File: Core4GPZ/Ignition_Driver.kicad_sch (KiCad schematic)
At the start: 8 parts, among them Q1 IRF740, Q2 IRF740

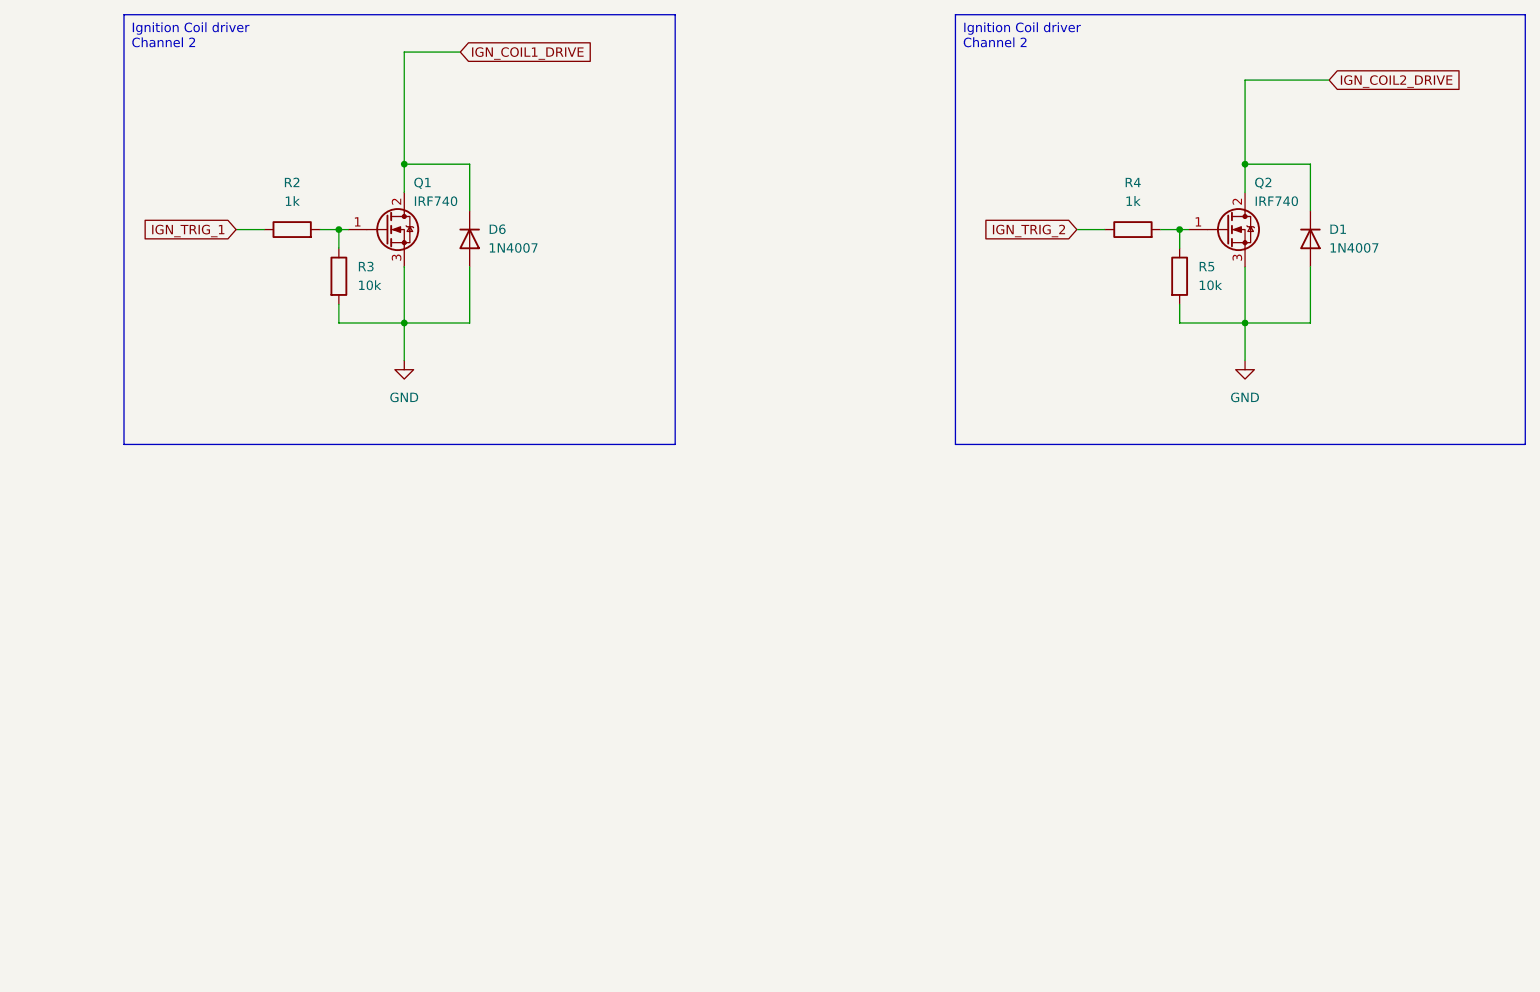
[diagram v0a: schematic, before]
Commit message: Test montage générateur de Haute tension
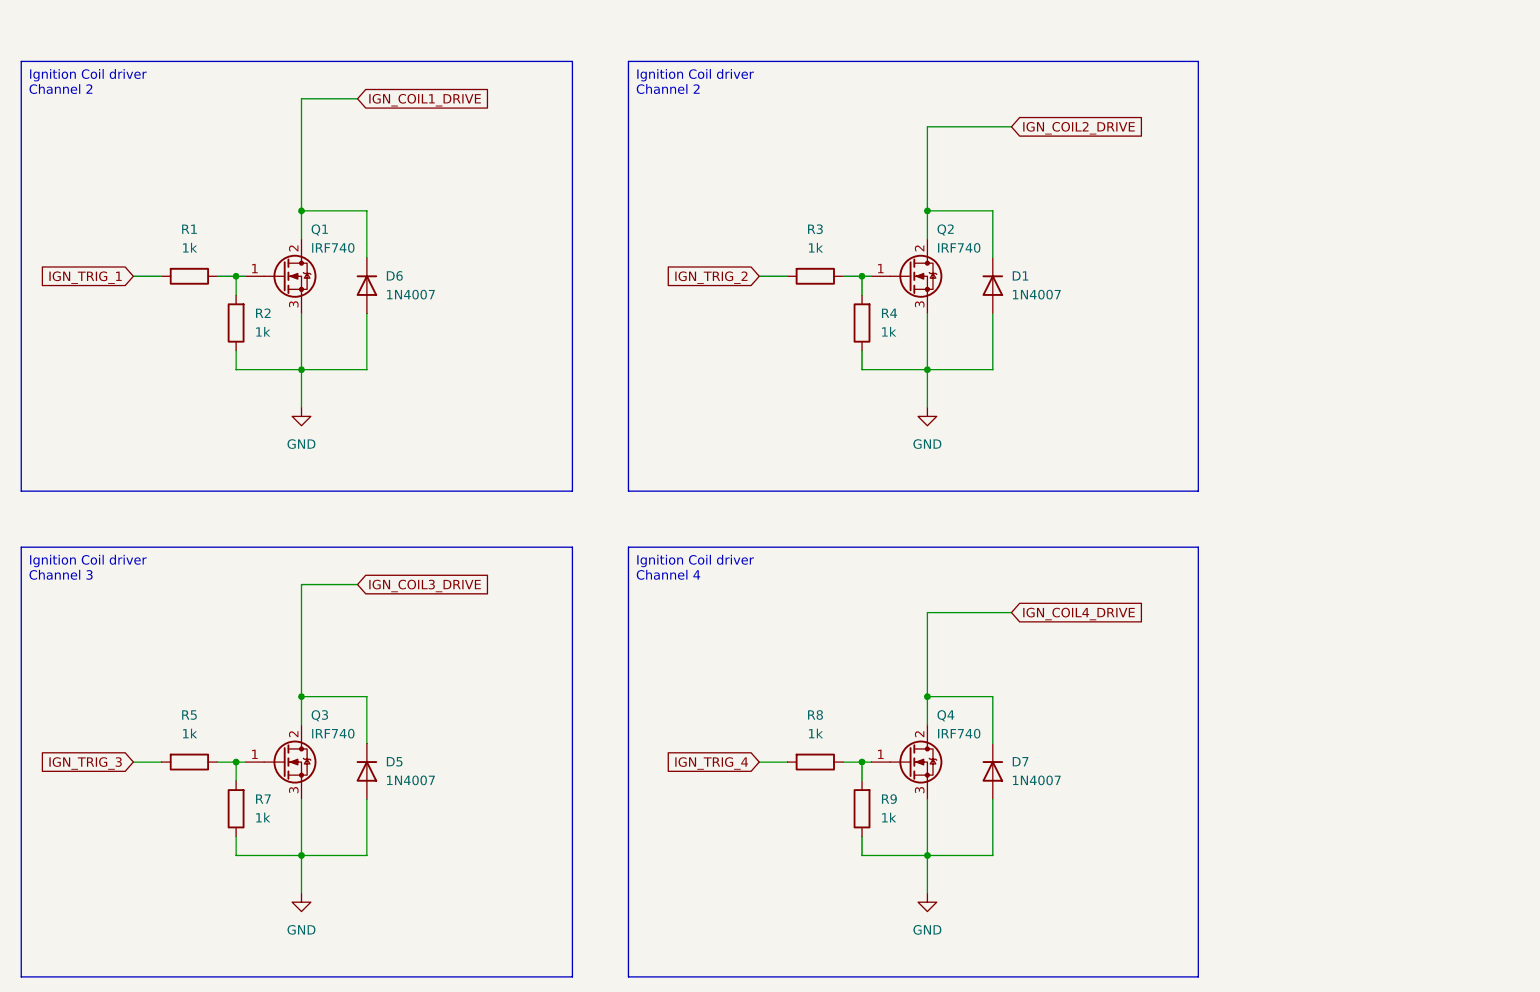
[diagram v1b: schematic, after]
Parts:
- added D5, D7: 1N4007, Diode_SMD:D_1206_3216Metric_Pad1.42x1.75mm_HandSolder, symbol Device:D
- added Q3, Q4: IRF740, Package_TO_SOT_THT:TO-220-3_Vertical, symbol Transistor_FET:IRF740
- added R1, R7, R8, R9: 1k, Resistor_SMD:R_0805_2012Metric_Pad1.20x1.40mm_HandSolder, symbol Device:R
- D1, D6: footprint Diode_THT:D_A-405_P2.54mm_Vertical_AnodeUp -> Diode_SMD:D_1206_3216Metric_Pad1.42x1.75mm_HandSolder
- R2, R4: footprint Resistor_THT:R_Axial_DIN0207_L6.3mm_D2.5mm_P10.16mm_Horizontal -> Resistor_SMD:R_0805_2012Metric_Pad1.20x1.40mm_HandSolder
- R3, R5: value 10k -> 1k; footprint Resistor_THT:R_Axial_DIN0207_L6.3mm_D2.5mm_P10.16mm_Horizontal -> Resistor_SMD:R_0805_2012Metric_Pad1.20x1.40mm_HandSolder
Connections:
- net GND: now also R2.1, R4.1, D5.2 (A), D7.2 (A), Q3.3 (S), Q4.3 (S), R7.1, R9.1; no longer R3.2, R5.2
- net IGN_TRIG_1: now also R1.2; no longer R2.1
- net IGN_TRIG_2: now also R3.2; no longer R4.1
- net at Q2.1 (G), R4.2: now also R3.1; no longer R5.1
- net at Q1.1 (G), R2.2: now also R1.1; no longer R3.1
- new net: Q3.1 (G), R5.1, R7.2
- new net: Q4.1 (G), R8.1, R9.2
- new net IGN_COIL3_DRIVE: D5.1 (K), Q3.2 (D)
- new net IGN_COIL4_DRIVE: D7.1 (K), Q4.2 (D)
- new net IGN_TRIG_3: R5.2
- new net IGN_TRIG_4: R8.2
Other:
- moved on the sheet: D6, Q1, Q2, R2
